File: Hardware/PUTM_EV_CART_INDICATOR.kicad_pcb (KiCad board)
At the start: 2 copper layers, 43 x 27 mm, 19 parts, among them J1 Screw_Terminal_01x08, K3 IM07DTS, K4 IM07DTS

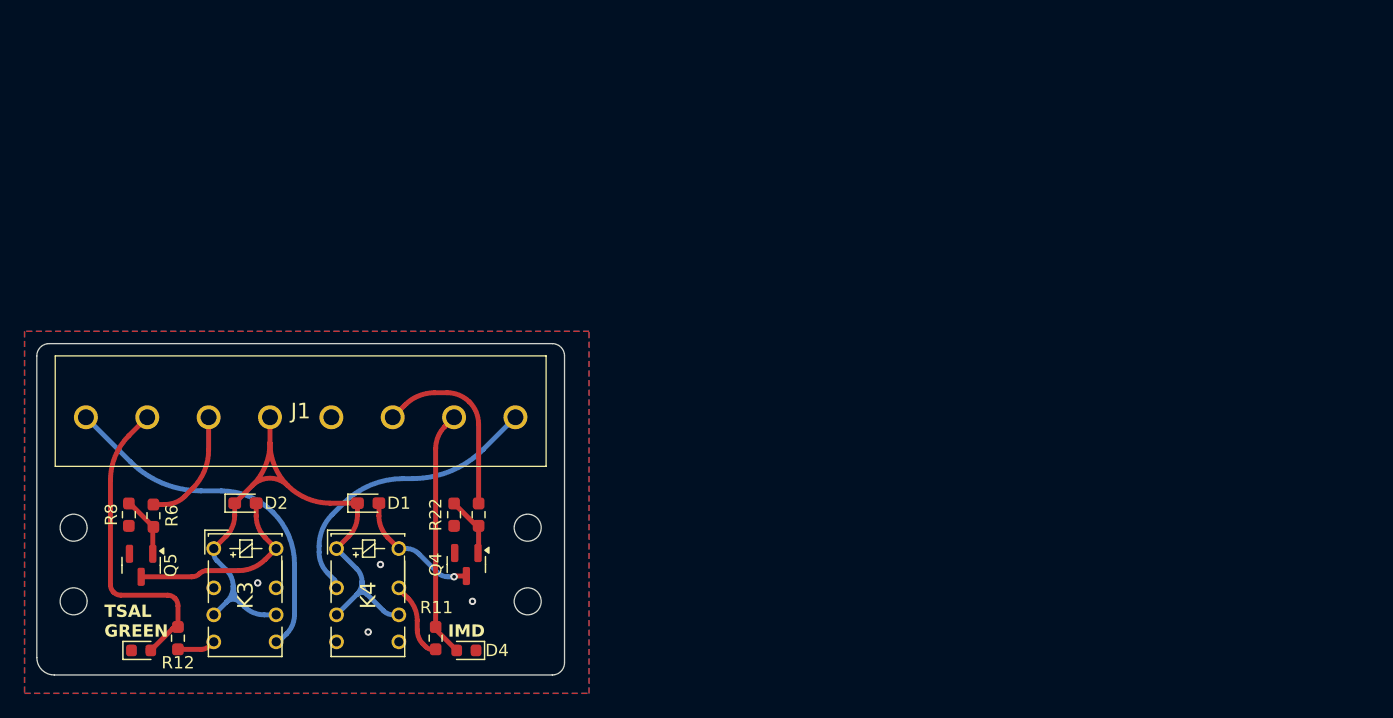
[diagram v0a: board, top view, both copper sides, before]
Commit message: Wersja 2.0 do sprawdzenia :3
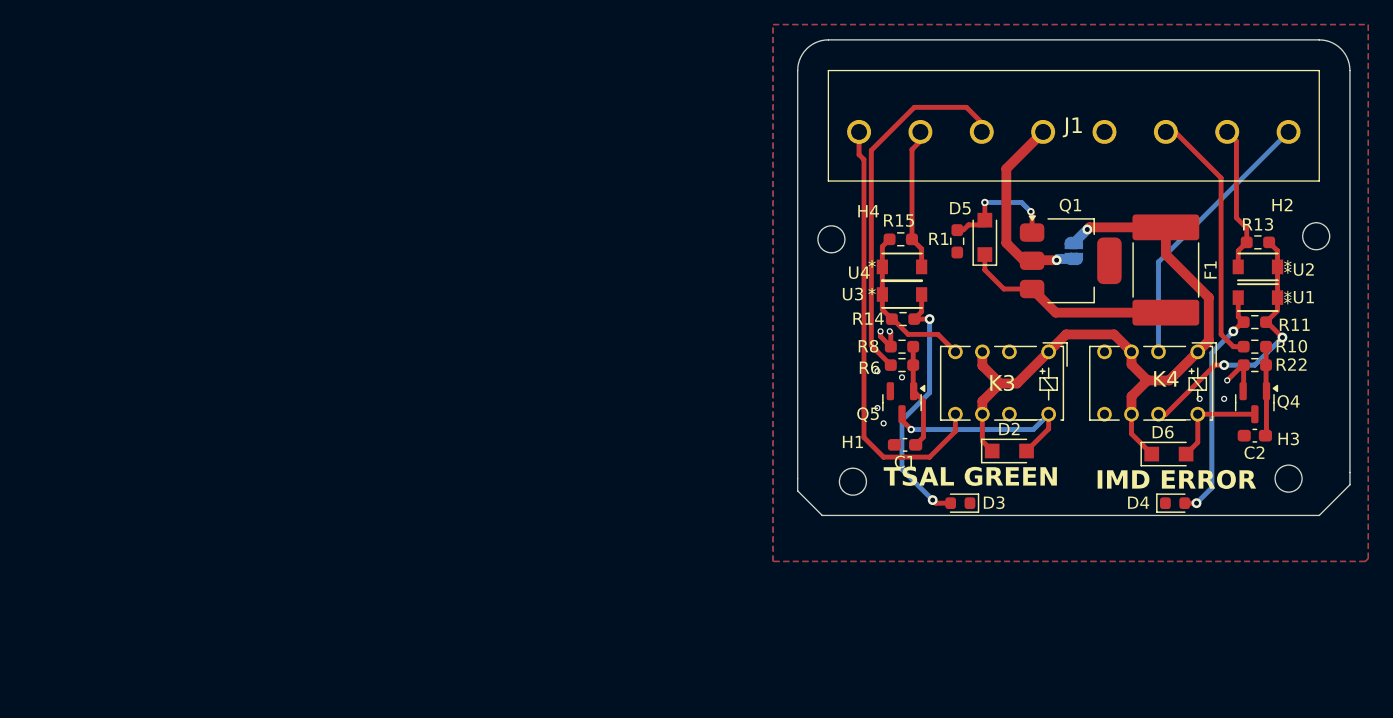
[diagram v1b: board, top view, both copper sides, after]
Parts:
- removed D1: D, Diode_SMD:D_0603_1608Metric_Pad1.05x0.95mm_HandSolder
- removed the H1 at (122.0, 80.0)
- removed the H1 at (85.0, 80.0)
- removed the H2 at (122.0, 74.0)
- removed the H2 at (85.0, 74.0)
- removed R12: 1K, Resistor_SMD:R_0603_1608Metric_Pad0.98x0.95mm_HandSolder
- added C1: NC, Capacitor_SMD:C_0603_1608Metric_Pad1.08x0.95mm_HandSolder, F.Cu at (152.8, 67.2)
- added C2: NC, Capacitor_SMD:C_0603_1608Metric_Pad1.08x0.95mm_HandSolder, F.Cu at (181.2, 66.5)
- added D5: D, Diode_SMD:Nexperia_CFP3_SOD-123W, F.Cu at (159.2, 50.3)
- added D6: D, Diode_SMD:Nexperia_CFP3_SOD-123W, F.Cu at (174.2, 68.0)
- added F1: 1.5A PPTC fuse, Library:Fuse_2920_7451Metric_Pad2.10x5.45mm_HandSolder, F.Cu at (174.0, 53.0)
- added H1: MountingHole, MountingHole:MountingHole_2.2mm_M2, F.Cu at (148.5, 70.2)
- added H2: MountingHole, MountingHole:MountingHole_2.2mm_M2, F.Cu at (186.2, 50.2)
- added H3: MountingHole, MountingHole:MountingHole_2.2mm_M2, F.Cu at (184.0, 70.0)
- added H4: MountingHole, MountingHole:MountingHole_2.2mm_M2, F.Cu at (146.8, 50.5)
- added JP1: Jumper_2_Open, Jumper:SolderJumper-2_P1.3mm_Open_RoundedPad1.0x1.5mm, B.Cu at (166.5, 51.5)
- added Q1: PMOS, Package_TO_SOT_SMD:SOT-223, F.Cu at (166.2, 52.2)
- added R1: R_Small, Resistor_SMD:R_0603_1608Metric_Pad0.98x0.95mm_HandSolder, F.Cu at (157.0, 50.7)
- added R13: NC, Resistor_SMD:R_0603_1608Metric_Pad0.98x0.95mm_HandSolder, F.Cu at (181.5, 50.8)
- added R14: NC, Resistor_SMD:R_0603_1608Metric_Pad0.98x0.95mm_HandSolder, F.Cu at (152.6, 57.0)
- added R15: NC, Resistor_SMD:R_0603_1608Metric_Pad0.98x0.95mm_HandSolder, F.Cu at (152.4, 50.5)
- added U1: 30mA const current led driver, Include:DIO_1-13_DIO-L, F.Cu at (181.5, 55.2)
- added U2: 30mA const current led driver, Include:DIO_1-13_DIO-L, F.Cu at (181.5, 52.8)
- added U3: 30mA const current led driver, Include:DIO_1-13_DIO-L, F.Cu at (152.5, 55.0)
- added U4: 30mA const current led driver, Include:DIO_1-13_DIO-L, F.Cu at (152.5, 52.8)
- D2: footprint Diode_SMD:D_0603_1608Metric_Pad1.05x0.95mm_HandSolder -> Diode_SMD:Nexperia_CFP3_SOD-123W
- R11: value 1K -> NC
- moved R11 71.5 mm to (181.2, 57.2), turned to 0 degrees
- moved D3 67.8 mm to (157.2, 72.0), turned to 180 degrees
- moved J1 67.2 mm to (149.0, 41.8)
- moved R22 66.4 mm to (181.2, 60.8), turned to 180 degrees
- moved K4 66.1 mm to (172.8, 62.2), turned to 180 degrees
- moved Q4 65.6 mm to (181.2, 63.8)
- moved R10 64.7 mm to (181.2, 59.2), turned to 180 degrees
- moved R8 64.5 mm to (152.5, 59.2), turned to 0 degrees
- moved K3 64.0 mm to (160.7, 62.2), turned to 180 degrees
- moved Q5 63.4 mm to (152.5, 63.8)
- moved D2 62.4 mm to (161.2, 67.8)
- moved R6 62.2 mm to (152.5, 60.8), turned to 180 degrees
- moved D4 59.0 mm to (174.8, 72.0), turned to 0 degrees
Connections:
- net Net-(K4-NC_2) renamed /current_driver/Input
- D2 pad 1: +24V -> /24V_fused
- D3 pad 2: /TSAL_LED -> /current_driver2/Output
- D4 pad 2: /IMD_LED -> /current_driver/Output
- K3 pad 1: +24V -> /24V_fused
- K3 pad 3: +24V -> /24V_fused
- K3 pad 4: Net-(K3-NO_1) -> /current_driver2/Input
- K3 pad 6: +24V -> /24V_fused
- K4 pad 1: +24V -> /24V_fused
- K4 pad 3: +24V -> /24V_fused
- K4 pad 6: +24V -> /24V_fused
- R11 pad 1: /IMD_LED -> /current_driver/Output
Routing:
- net /24V_fused: track 0.00 -> 58.0 mm, vias 0 -> 1
- net +24V: track 54.2 -> 16.5 mm, vias 0 -> 1
- net /current_driver2/Output: track 0.00 -> 21.8 mm, vias 0 -> 2
- net /TSAL_GREEN: track 9.76 -> 29.9 mm
- net /current_driver/Output: track 0.00 -> 19.5 mm, vias 0 -> 2
- net Net-(D5-K): track 0.00 -> 18.0 mm
- net /current_driver/Input: track 6.36 -> 22.0 mm, vias 0 -> 2
- net /current_driver2/Input: track 0.00 -> 13.7 mm
- net /TSAL_LED: track 25.8 -> 12.4 mm
- net Net-(D5-A): track 0.00 -> 9.17 mm, vias 0 -> 2
- net /IMD_LED: track 20.2 -> 11.9 mm
- net GND: track 0.00 -> 6.88 mm, vias 4 -> 9
- net /TSAL_COLUMN: track 29.4 -> 36.2 mm
- net /IMD: track 15.6 -> 21.1 mm
- net Net-(Q5-G): track 4.97 -> 8.61 mm
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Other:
- board size 43 x 27 mm -> 45 x 38.8 mm
- board text added: "IMD ERROR"
- board text removed: "IMD"
- board text removed: "Krzysiu Ch*** faktury oddawaj"
